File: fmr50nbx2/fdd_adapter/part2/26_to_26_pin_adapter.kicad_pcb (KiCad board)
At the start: 2 copper layers, 99.7 x 11 mm, 2 parts, among them J1 Conn_01x26_Female, J2 Conn_01x26_Female

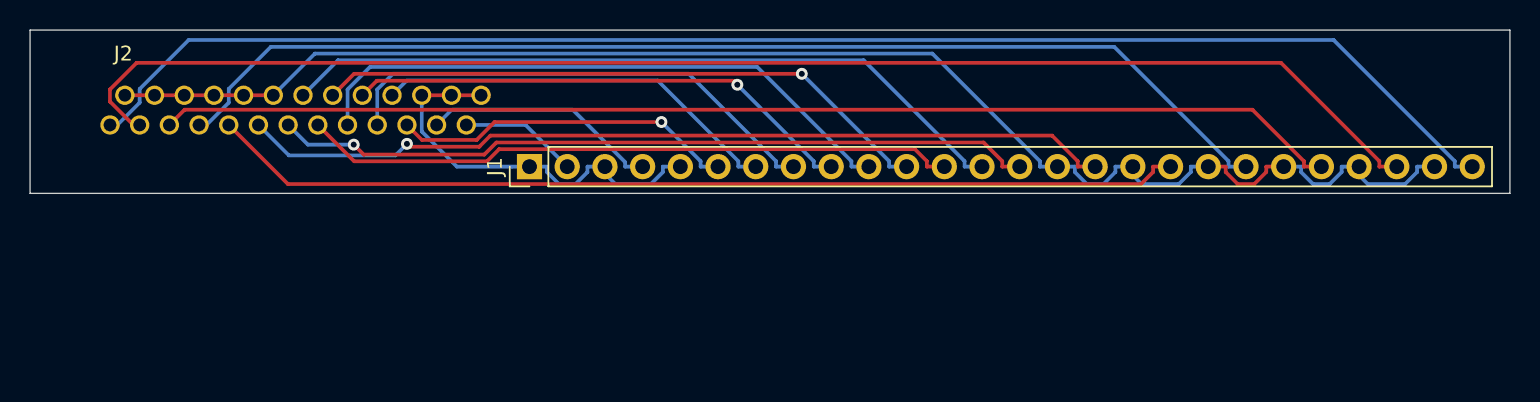
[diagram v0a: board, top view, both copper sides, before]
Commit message: Add files via upload
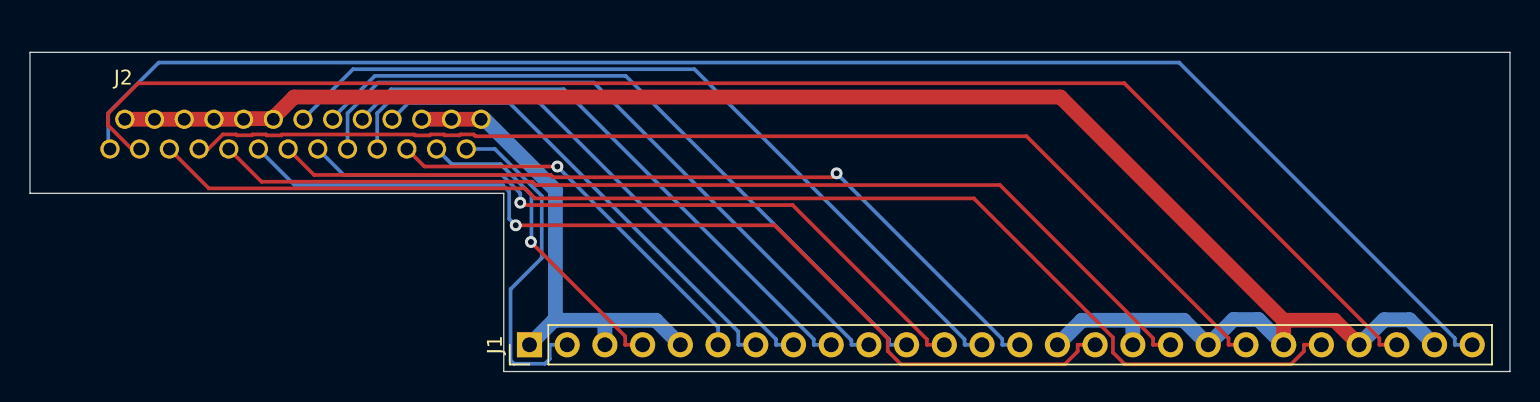
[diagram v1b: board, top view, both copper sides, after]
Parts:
- moved J1 12.0 mm to (68.8, 76.2)
- moved J2 1.62 mm to (40.6, 65.7)
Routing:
- net GND: track 100.5 -> 118.5 mm
- net Net-(J1-Pad2): track 7.96 -> 23.3 mm
- net Net-(J1-Pad16): track 59.0 -> 64.7 mm
- net Net-(J1-Pad11): track 42.1 -> 47.6 mm, vias 1 -> 0
- net Net-(J1-Pad4): track 16.1 -> 21.6 mm, vias 0 -> 1
- net Net-(J1-Pad26): track 98.4 -> 103.9 mm
- net Net-(J1-Pad9): track 34.6 -> 39.8 mm, vias 1 -> 0
- net Net-(J1-Pad22): track 79.8 -> 85.0 mm
- net Net-(J1-Pad13): track 49.9 -> 55.0 mm
- net VCC: track 27.9 -> 32.9 mm
- net Net-(J1-Pad24): track 94.0 -> 98.8 mm
- net Net-(J1-Pad10): track 41.1 -> 45.9 mm
- net Net-(J1-Pad7): track 27.5 -> 32.2 mm
- net Net-(J1-Pad8): track 33.7 -> 38.1 mm
- net Net-(J1-Pad12): track 44.3 -> 48.2 mm, vias 0 -> 1
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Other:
- board size 99.7 x 11 mm -> 99.7 x 21.5 mm
